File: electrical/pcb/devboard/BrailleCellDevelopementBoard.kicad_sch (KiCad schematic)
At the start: 5 parts, among them J2 USB_C_Receptacle_USB2.0_14P, Q3 PMOS

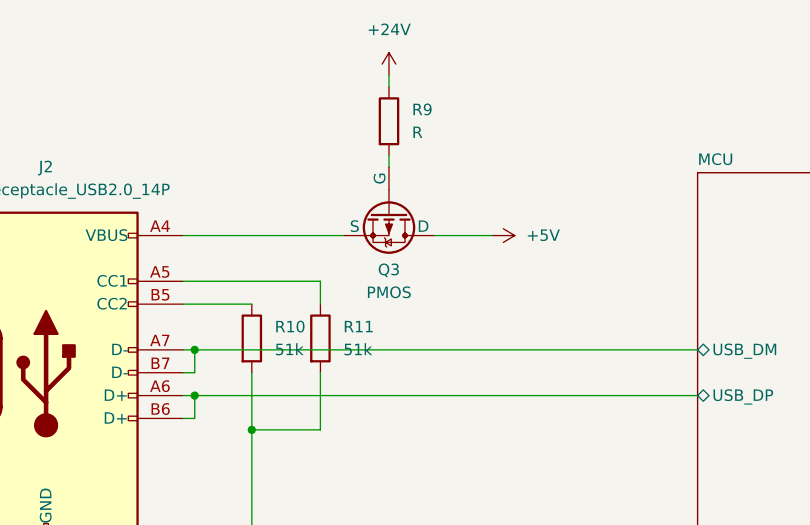
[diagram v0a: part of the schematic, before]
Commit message: Add files via upload
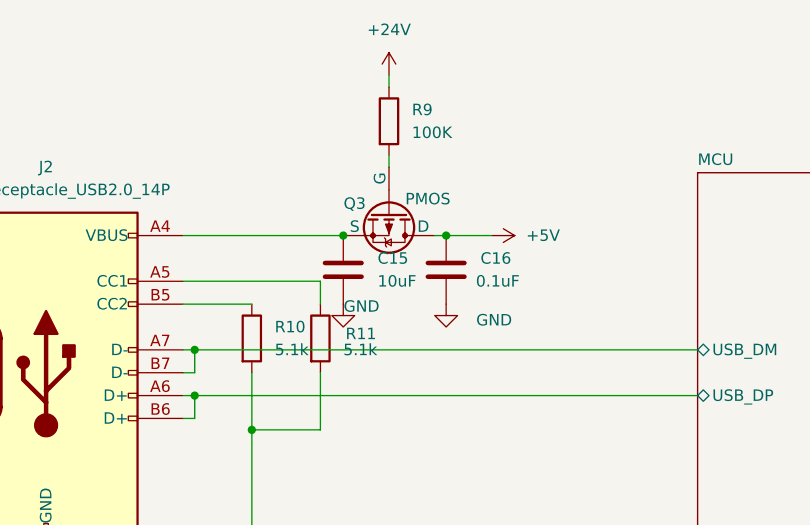
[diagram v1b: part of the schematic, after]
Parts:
- added C15: 10uF, Capacitor_SMD:C_0603_1608Metric, symbol Device:C
- added C16: 0.1uF, Capacitor_SMD:C_0603_1608Metric, symbol Device:C
- J2: footprint (none) -> Connector_USB:USB_C_Receptacle_GCT_USB4085
- Q3: footprint (none) -> Package_SO:SO-8_3.9x4.9mm_P1.27mm
- R10, R11: value 51k -> 5.1k; footprint (none) -> Resistor_SMD:R_0603_1608Metric
- R9: value R -> 100K; footprint (none) -> Resistor_SMD:R_0603_1608Metric
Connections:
- net +5V: now also C16.1
- net GND: now also C15.2, C16.2
- net at J2.A4 (VBUS), J2.A9 (VBUS), J2.B4 (VBUS)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: now also C15.1
